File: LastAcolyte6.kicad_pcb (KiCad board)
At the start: 4 copper layers, 100 x 100 mm, 87 parts, among them J1 Conn_02x23_Odd_Even, J10 DualPower_USB_B, J11 Conn_01x06, J2 DE9_Plug, J3 Conn_02x05_Odd_Even, J4 DE9_Plug, J5 DE15_Receptacle_HighDensity, J6 AudioJack3, J7 Mini-DIN-6, J8 Mini-DIN-6, J9 Micro_SD_Card, SW1 SW_Push, SW2 SW_SPDT, U1 XC9572VQ44, U10 74AHCT245, U11 74AHCT245, U12 74AHCT08, U15 74AHCT245, U16 74AHCT245, U19 74AHCT374, U2 IS61C5128AL-10KLI, U21 PIC16F886-IP, U3 LM1117MP-3.3, U4 W65C816SxQ, U5 W65C22SxQ, U6 74AHCT273, U7 IS61C5128AL-10KLI, U8 74HCT166, U9 74HCT166, X1 CXO_DIP8

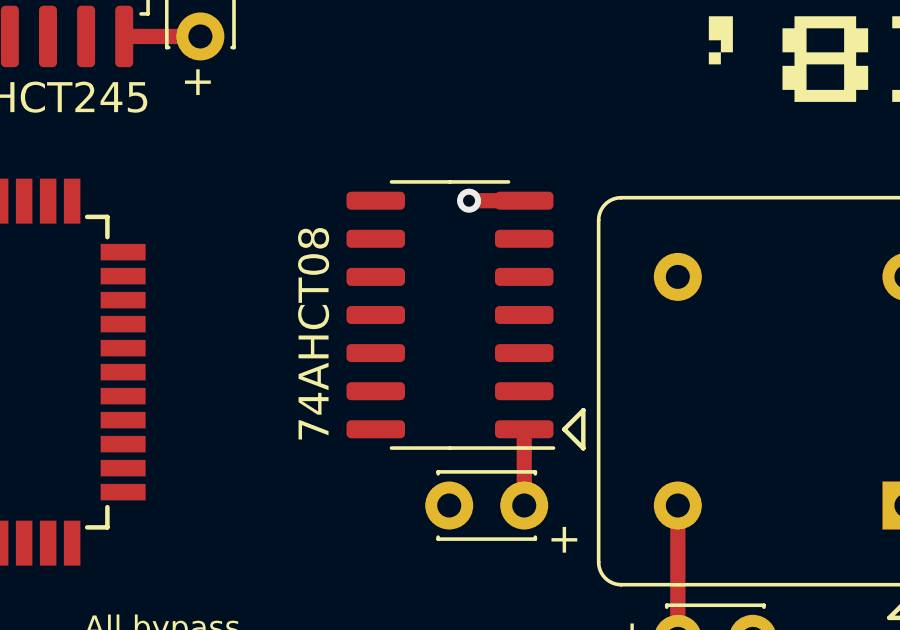
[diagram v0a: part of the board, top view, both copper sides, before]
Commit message: Add files via upload
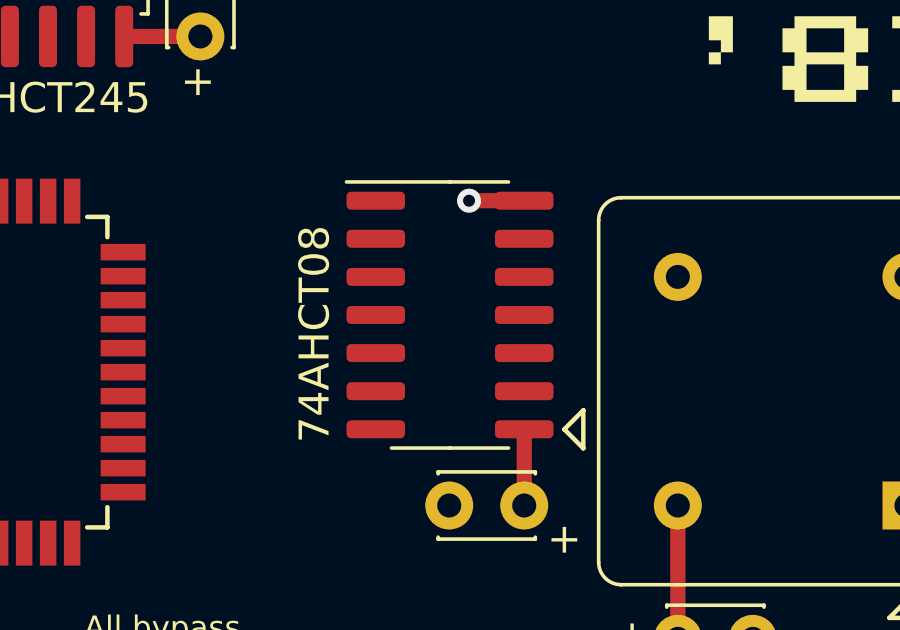
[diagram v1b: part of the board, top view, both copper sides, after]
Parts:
- turned U12 to 0 degrees
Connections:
- U12 pad 10: unconnected-(U12-Pad10) -> PHI2-3V3
- U12 pad 11: unconnected-(U12-Pad11) -> WHITE-PIX-B
- U12 pad 12: unconnected-(U12-Pad12) -> TEXT-PIX-B
- U12 pad 13: unconnected-(U12-Pad13) -> ~{PHI2-3V3}
- U12 pad 2: ~{PHI2-3V3} -> PHI2-3V3
- U12 pad 5: VIA-3V3 -> ~{VIA-3V3}
- U12 pad 8: unconnected-(U12-Pad8) -> WHITE-PIX-A
- U12 pad 9: unconnected-(U12-Pad9) -> TEXT-PIX-A
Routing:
- net GND: track 37.7 -> 35.8 mm, vias 18 -> 17
- net +5V: track 79.6 -> 81.4 mm, vias 0 -> 1

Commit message: Add files via upload
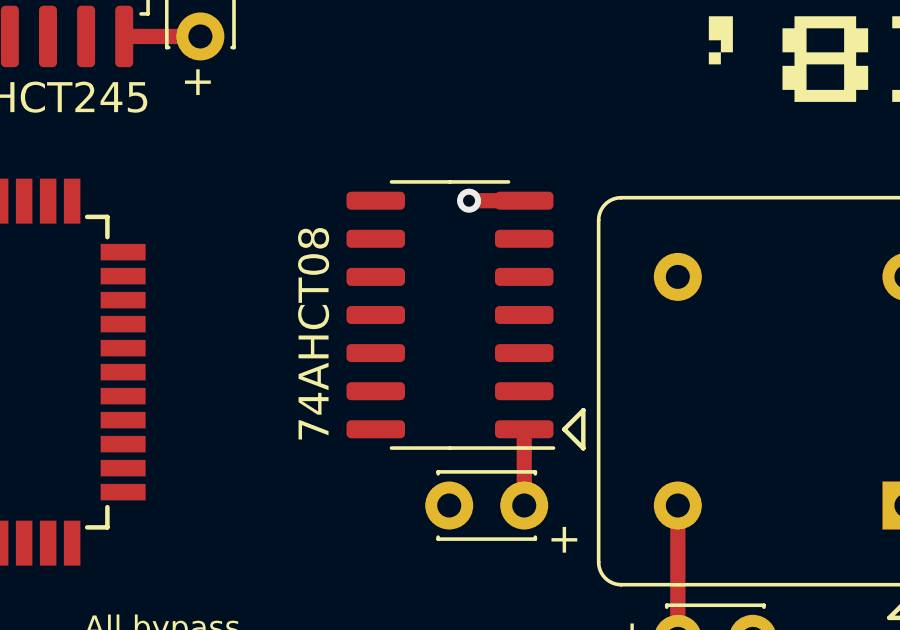
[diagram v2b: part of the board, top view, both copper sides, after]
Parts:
- turned U12 to 180 degrees
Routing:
- net GND: track 35.8 -> 37.7 mm, vias 17 -> 18
- net +5V: track 81.4 -> 79.6 mm, vias 1 -> 0
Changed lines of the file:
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@@
   )
   (footprint "Package_SO:SOIC-14_3.9x8.7mm_P1.27mm" (layer "F.Cu")
-    (at 103.57 120.65)
+    (at 103.57 120.65 180)
     (descr "SOIC, 14 Pin (JEDEC MS-012AB, https://www.analog.com/media/en/package-pcb-resources/package/pkg_pdf/soic_narrow-r/r_14.pdf), generated with kicad-footprint-generator ipc_gullwing_generator.py")
     (tags "SOIC SO")
@@
         (effects (font (size 1 1) (thickness 0.15)))
     )
-    (fp_text user "74AHCT08" (at -4.51 0.635 90 unlocked) (layer "F.SilkS")
+    (fp_text user "74AHCT08" (at 4.51 -0.635 90 unlocked) (layer "F.SilkS")
         (effects (font (size 1 1) (thickness 0.15)))
     )
@@
     (fp_line (start 1.95 4.325) (end -1.95 4.325)
       (stroke (width 0.1) (type solid)) (layer "F.Fab"))
-    (pad "1" smd roundrect (at -2.475 -3.81) (size 1.95 0.6) (layers "F.Cu" "F.Paste" "F.Mask") (roundrect_rratio 0.25)
+    (pad "1" smd roundrect (at -2.475 -3.81 180) (size 1.95 0.6) (layers "F.Cu" "F.Paste" "F.Mask") (roundrect_rratio 0.25)
       (net 1 "+5V") (pintype "input"))
-    (pad "2" smd roundrect (at -2.475 -2.54) (size 1.95 0.6) (layers "F.Cu" "F.Paste" "F.Mask") (roundrect_rratio 0.25)
+    (pad "2" smd roundrect (at -2.475 -2.54 180) (size 1.95 0.6) (layers "F.Cu" "F.Paste" "F.Mask") (roundrect_rratio 0.25)
       (net 57 "PHI2-3V3") (pintype "input"))
-    (pad "3" smd roundrect (at -2.475 -1.27) (size 1.95 0.6) (layers "F.Cu" "F.Paste" "F.Mask") (roundrect_rratio 0.25)
+    (pad "3" smd roundrect (at -2.475 -1.27 180) (size 1.95 0.6) (layers "F.Cu" "F.Paste" "F.Mask") (roundrect_rratio 0.25)
       (net 129 "PHI2") (pintype "output"))
-    (pad "4" smd roundrect (at -2.475 0) (size 1.95 0.6) (layers "F.Cu" "F.Paste" "F.Mask") (roundrect_rratio 0.25)
+    (pad "4" smd roundrect (at -2.475 0 180) (size 1.95 0.6) (layers "F.Cu" "F.Paste" "F.Mask") (roundrect_rratio 0.25)
       (net 1 "+5V") (pintype "input"))
-    (pad "5" smd roundrect (at -2.475 1.27) (size 1.95 0.6) (layers "F.Cu" "F.Paste" "F.Mask") (roundrect_rratio 0.25)
+    (pad "5" smd roundrect (at -2.475 1.27 180) (size 1.95 0.6) (layers "F.Cu" "F.Paste" "F.Mask") (roundrect_rratio 0.25)
       (net 174 "~{VIA-3V3}") (pintype "input"))
-    (pad "6" smd roundrect (at -2.475 2.54) (size 1.95 0.6) (layers "F.Cu" "F.Paste" "F.Mask") (roundrect_rratio 0.25)
+    (pad "6" smd roundrect (at -2.475 2.54 180) (size 1.95 0.6) (layers "F.Cu" "F.Paste" "F.Mask") (roundrect_rratio 0.25)
       (net 131 "~{VIA}") (pintype "output"))
-    (pad "7" smd roundrect (at -2.475 3.81) (size 1.95 0.6) (layers "F.Cu" "F.Paste" "F.Mask") (roundrect_rratio 0.25)
+    (pad "7" smd roundrect (at -2.475 3.81 180) (size 1.95 0.6) (layers "F.Cu" "F.Paste" "F.Mask") (roundrect_rratio 0.25)
       (net 2 "GND") (pinfunction "GND") (pintype "power_in"))
-    (pad "8" smd roundrect (at 2.475 3.81) (size 1.95 0.6) (layers "F.Cu" "F.Paste" "F.Mask") (roundrect_rratio 0.25)
+    (pad "8" smd roundrect (at 2.475 3.81 180) (size 1.95 0.6) (layers "F.Cu" "F.Paste" "F.Mask") (roundrect_rratio 0.25)
       (net 51 "WHITE-PIX-A") (pintype "output"))
-    (pad "9" smd roundrect (at 2.475 2.54) (size 1.95 0.6) (layers "F.Cu" "F.Paste" "F.Mask") (roundrect_rratio 0.25)
+    (pad "9" smd roundrect (at 2.475 2.54 180) (size 1.95 0.6) (layers "F.Cu" "F.Paste" "F.Mask") (roundrect_rratio 0.25)
       (net 52 "TEXT-PIX-A") (pintype "input"))
-    (pad "10" smd roundrect (at 2.475 1.27) (size 1.95 0.6) (layers "F.Cu" "F.Paste" "F.Mask") (roundrect_rratio 0.25)
+    (pad "10" smd roundrect (at 2.475 1.27 180) (size 1.95 0.6) (layers "F.Cu" "F.Paste" "F.Mask") (roundrect_rratio 0.25)
       (net 57 "PHI2-3V3") (pintype "input"))
-    (pad "11" smd roundrect (at 2.475 0) (size 1.95 0.6) (layers "F.Cu" "F.Paste" "F.Mask") (roundrect_rratio 0.25)
+    (pad "11" smd roundrect (at 2.475 0 180) (size 1.95 0.6) (layers "F.Cu" "F.Paste" "F.Mask") (roundrect_rratio 0.25)
       (net 53 "WHITE-PIX-B") (pintype "output"))
-    (pad "12" smd roundrect (at 2.475 -1.27) (size 1.95 0.6) (layers "F.Cu" "F.Paste" "F.Mask") (roundrect_rratio 0.25)
+    (pad "12" smd roundrect (at 2.475 -1.27 180) (size 1.95 0.6) (layers "F.Cu" "F.Paste" "F.Mask") (roundrect_rratio 0.25)
       (net 54 "TEXT-PIX-B") (pintype "input"))
-    (pad "13" smd roundrect (at 2.475 -2.54) (size 1.95 0.6) (layers "F.Cu" "F.Paste" "F.Mask") (roundrect_rratio 0.25)
+    (pad "13" smd roundrect (at 2.475 -2.54 180) (size 1.95 0.6) (layers "F.Cu" "F.Paste" "F.Mask") (roundrect_rratio 0.25)
       (net 58 "~{PHI2-3V3}") (pintype "input"))
-    (pad "14" smd roundrect (at 2.475 -3.81) (size 1.95 0.6) (layers "F.Cu" "F.Paste" "F.Mask") (roundrect_rratio 0.25)
+    (pad "14" smd roundrect (at 2.475 -3.81 180) (size 1.95 0.6) (layers "F.Cu" "F.Paste" "F.Mask") (roundrect_rratio 0.25)
       (net 1 "+5V") (pinfunction "VCC") (pintype "power_in"))
     (model "${KICAD6_3DMODEL_DIR}/Package_SO.3dshapes/SOIC-14_3.9x8.7mm_P1.27mm.wrl"
@@
   (segment (start 111.265 149.21) (end 111.265 152.3) (width 0.508) (layer "F.Cu") (net 1))
   (segment (start 137.795 153.275) (end 135.255 153.275) (width 0.508) (layer "F.Cu") (net 1))
-  (segment (start 106.045 116.84) (end 104.205 116.84) (width 0.508) (layer "F.Cu") (net 1))
   (segment (start 111.165 127) (end 111.165 131.445) (width 0.508) (layer "F.Cu") (net 1))
   (segment (start 71.755 121.92) (end 74.95 121.92) (width 0.508) (layer "F.Cu") (net 1))
@@
   (segment (start 127 104.775) (end 127 102.235) (width 0.508) (layer "F.Cu") (net 1))
   (segment (start 92.71 111.365) (end 95.25 111.365) (width 0.508) (layer "F.Cu") (net 1))
-  (via (at 104.205 116.84) (size 0.8) (drill 0.4) (layers "F.Cu" "B.Cu") (net 1))
   (segment (start 117.475 143.129) (end 117.894 142.71) (width 0.508) (layer "F.Cu") (net 2))
   (segment (start 152.02 100.965) (end 150.495 100.965) (width 0.508) (layer "F.Cu") (net 2))
@@
   (segment (start 123.825 145.175) (end 123.825 146.925) (width 0.508) (layer "F.Cu") (net 2))
   (segment (start 116.065 89.375) (end 116.065 87.645) (width 0.508) (layer "F.Cu") (net 2))
+  (segment (start 106.045 116.84) (end 104.205 116.84) (width 0.508) (layer "F.Cu") (net 2))
   (segment (start 117.856 143.51) (end 119.365 143.51) (width 0.508) (layer "F.Cu") (net 2))
   (segment (start 117.495 93.345) (end 119.365 93.345) (width 0.508) (layer "F.Cu") (net 2))
@@
   (via (at 67.775 80.18) (size 0.8) (drill 0.4) (layers "F.Cu" "B.Cu") (net 2))
   (via (at 117.475 143.129) (size 0.8) (drill 0.4) (layers "F.Cu" "B.Cu") (net 2))
+  (via (at 104.205 116.84) (size 0.8) (drill 0.4) (layers "F.Cu" "B.Cu") (net 2))
   (via (at 133.35 126.365) (size 0.8) (drill 0.4) (layers "F.Cu" "B.Cu") (net 2))
   (via (at 133.35 90.805) (size 0.8) (drill 0.4) (layers "F.Cu" "B.Cu") (net 2))
@@
     )
   )
+  (group "" (id 23c33717-44c8-44e4-869e-f67908dbf0d1)
+    (members
+      02fdd237-94cf-4eeb-bfa9-ab855244a659
+      1bfe771c-de59-4802-ac1f-5bfe987c95c5
+      6c576b43-8160-4a72-bcb2-5ccc907c7545
+      6fbddc10-24b8-482b-9395-9df413870231
+      7b8bfaf1-8b7c-4401-9cd0-3c7fa825d7f4
+      a284555b-34f8-49ce-88a8-3128ece8b229
+      a5b50d78-a37b-4e9e-a5c7-f50ed3021f4c
+      afd4bacc-ac44-464f-9f35-001d38f8b7d5
+      df1c0b5e-bf36-4a59-ba09-69c21e3946a5
+    )
+  )
